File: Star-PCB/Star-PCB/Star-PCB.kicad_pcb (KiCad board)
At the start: 2 copper layers, 100 x 100 mm, 6 parts

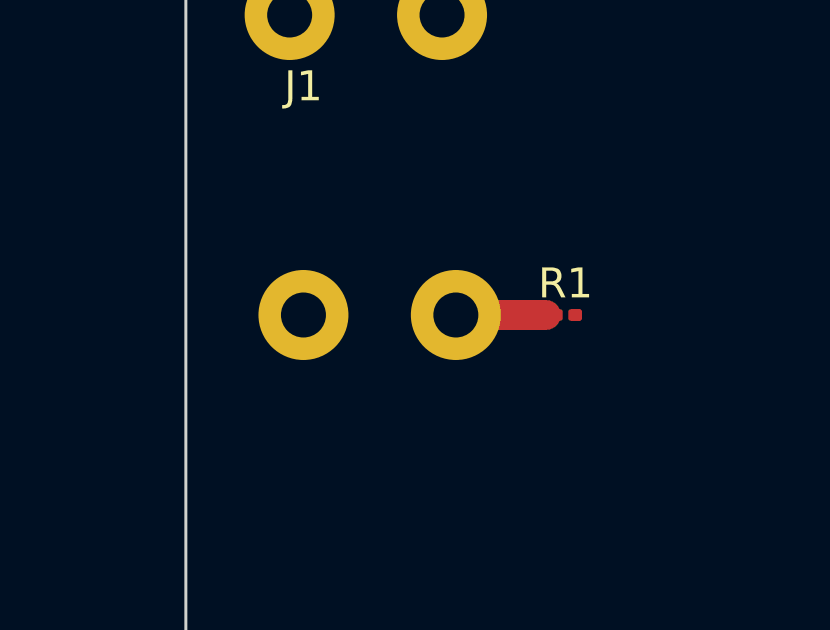
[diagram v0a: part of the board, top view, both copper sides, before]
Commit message: Fixed it
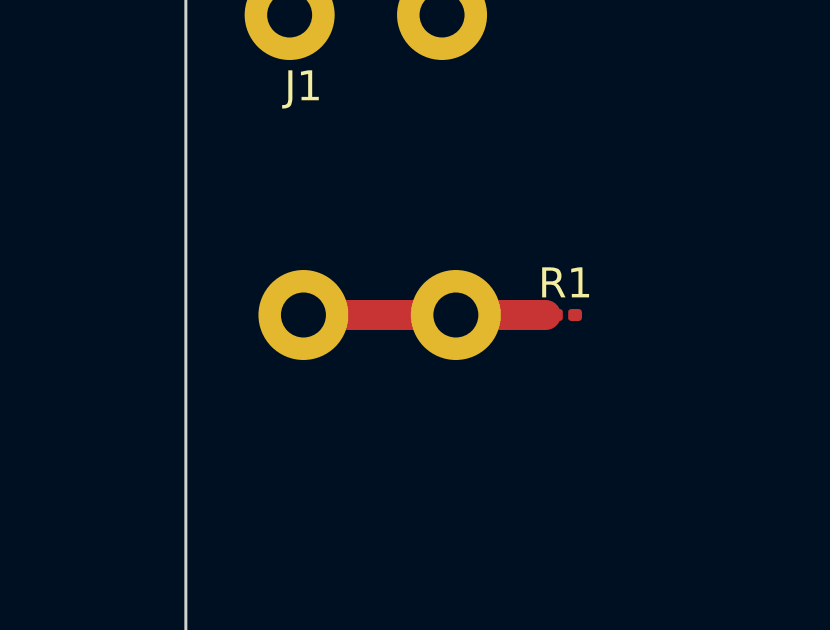
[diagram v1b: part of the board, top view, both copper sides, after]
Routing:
- net Net-(J1-Pad1): track 3.00 -> 8.08 mm
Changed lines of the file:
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@@
   (via (at 218 33) (size 0.8) (drill 0.4) (layers "F.Cu" "B.Cu") (free) (net 2))
   (via (at 133 33) (size 0.8) (drill 0.4) (layers "F.Cu" "B.Cu") (free) (net 2))
+  (segment (start 129 88) (end 123.92 88) (width 1) (layer "F.Cu") (net 9))
   (segment (start 129 88) (end 132 88) (width 1) (layer "F.Cu") (net 9))
   (zone (net 1) (net_name "Net-(D1-Pad1)") (layer "F.Cu") (hatch edge 0.5)

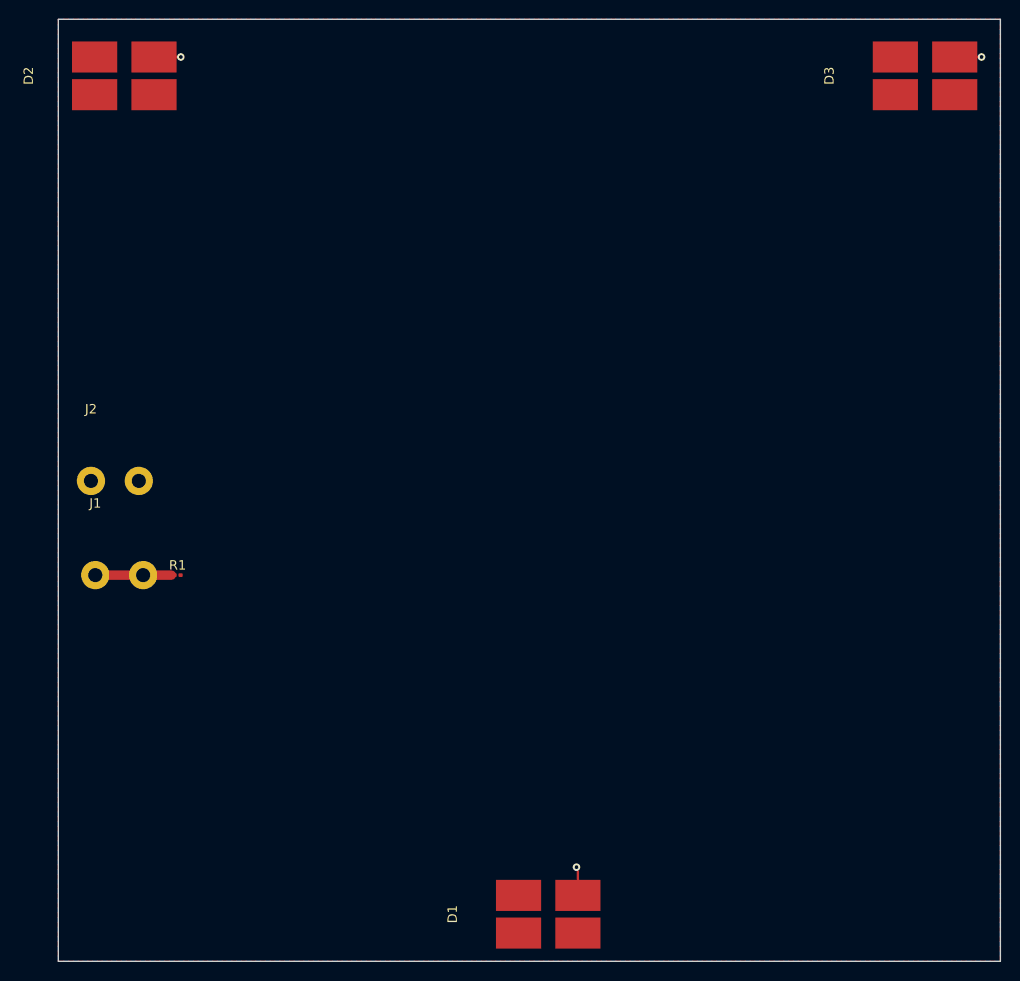
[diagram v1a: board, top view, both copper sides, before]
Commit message: DONE!
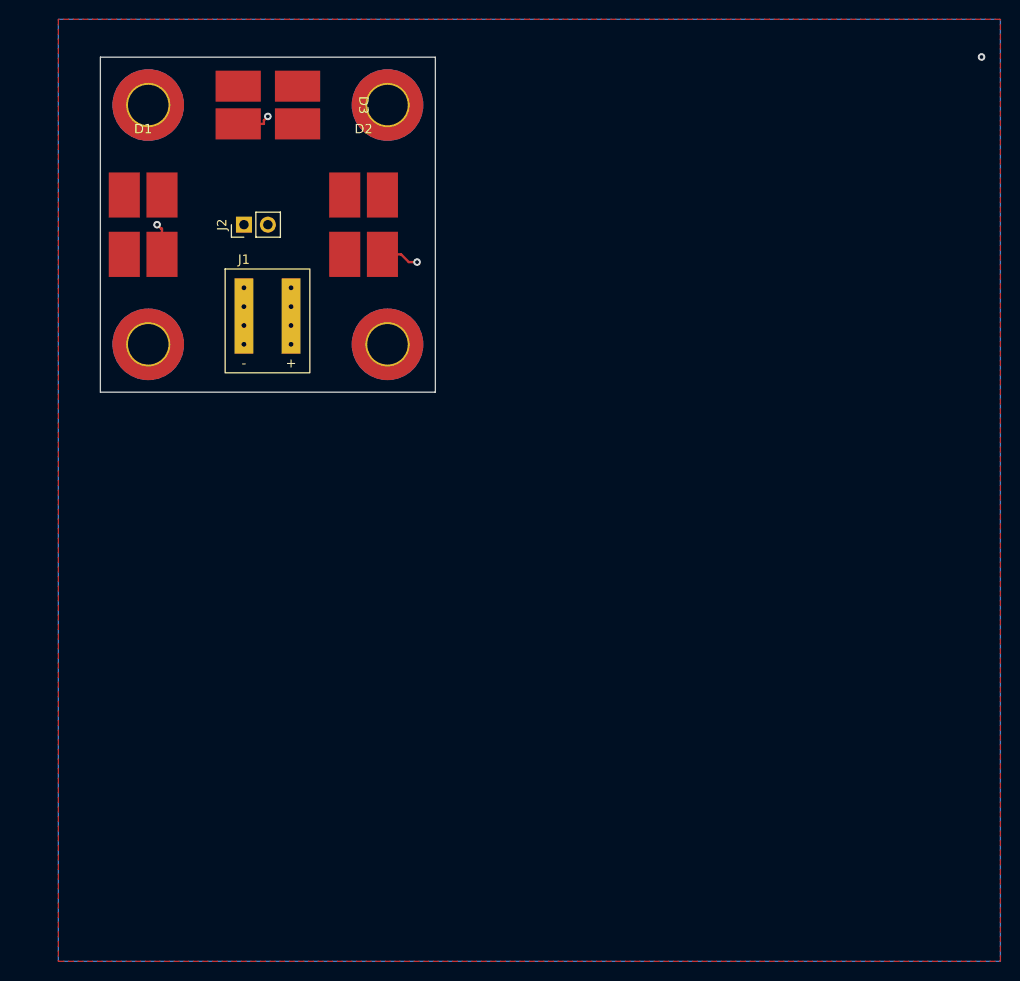
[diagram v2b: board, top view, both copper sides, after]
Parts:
- removed R1: ~, Resistor_SMD:R_0201_0603Metric
- added H1: MountingHole_Pad, MountingHole:MountingHole_4.3mm_M4_ISO7380_Pad_TopBottom, F.Cu at (129.5, 38.1)
- added H2: MountingHole_Pad, MountingHole:MountingHole_4.3mm_M4_ISO7380_Pad_TopBottom, F.Cu at (154.9, 38.1)
- added H3: MountingHole_Pad, MountingHole:MountingHole_4.3mm_M4_ISO7380_Pad_TopBottom, F.Cu at (154.9, 63.5)
- added H4: MountingHole_Pad, MountingHole:MountingHole_4.3mm_M4_ISO7380_Pad_TopBottom, F.Cu at (129.5, 63.5)
- J1: value ~ -> Conn_01x02; footprint Star-Library:EST026 -> Star-Library:star_connector
- J2: value ~ -> Conn_01x02; footprint Star-Library:EST026 -> Connector_PinHeader_2.54mm:PinHeader_1x02_P2.54mm_Vertical
- moved D1 84.9 mm to (129.0, 50.8), turned to 0 degrees
- moved D3 69.8 mm to (142.2, 38.1), turned to -90 degrees
- moved J1 34.4 mm to (141.7, 58.5)
- moved J2 31.7 mm to (139.7, 50.8), turned to 90 degrees
- moved D2 29.9 mm to (152.4, 50.8), turned to 0 degrees
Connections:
- D1 pad 1: Net-(D1-Pad1) -> Net-(J1-Pin_2)
- D1 pad 2: Net-(D1-Pad2) -> Net-(J1-Pin_1)
- D2 pad 1: Net-(D1-Pad1) -> Net-(J1-Pin_2)
- D2 pad 2: Net-(D1-Pad2) -> Net-(J1-Pin_1)
- D3 pad 1: Net-(D1-Pad1) -> Net-(J1-Pin_2)
- D3 pad 2: Net-(D1-Pad2) -> Net-(J1-Pin_1)
- J1 pad 1: Net-(J1-Pad1) -> Net-(J1-Pin_1)
- J2 pad 1: Net-(D1-Pad2) -> Net-(J1-Pin_1)
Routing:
- net Net-(J1-Pin_1): track 0.00 -> 11.1 mm, vias 0 -> 4
- net Net-(D1-Pad2): track 8.76 -> 0.00 mm, vias 3 -> 0
- net Net-(J1-Pad1): track 8.08 -> 0.00 mm
- net Net-(D1-Pad1): track 0.51 -> 0.00 mm
- added copper zone on B.Cu, net Net-(J1-Pin_1)
- added copper zone on F.Cu, net Net-(J1-Pin_2)
- removed copper zone on F.Cu, net Net-(D1-Pad1)
- removed copper zone on B.Cu, net Net-(D1-Pad2)
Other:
- board size 100 x 100 mm -> 35.6 x 35.6 mm
